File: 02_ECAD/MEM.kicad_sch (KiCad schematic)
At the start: 50 parts, among them U12 MT53E1G32D2FW-046_WT:A, U13 SDINBDG4-16G-I2, U14 IS25LP256D-JLLE

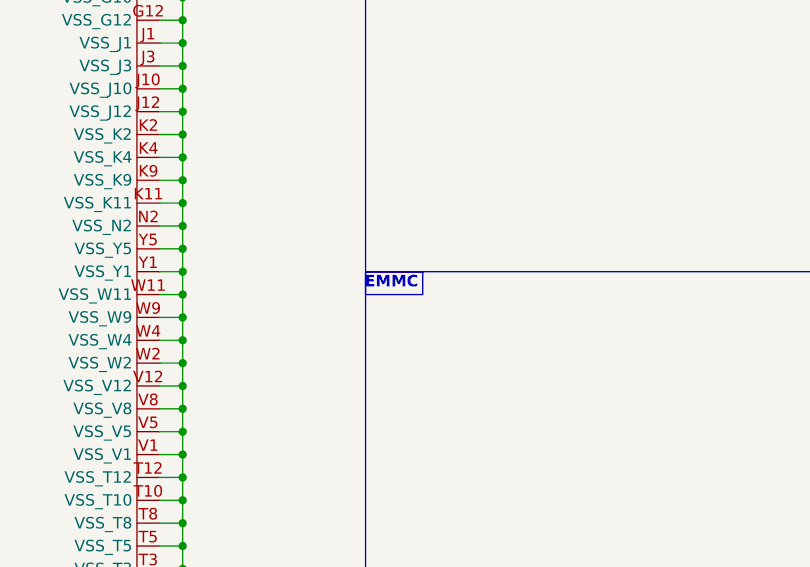
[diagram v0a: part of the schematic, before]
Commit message: Skew Check.
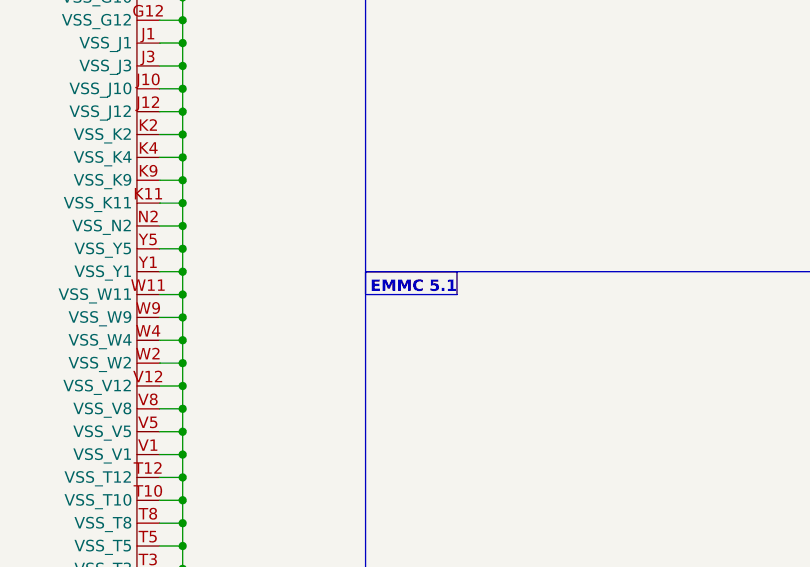
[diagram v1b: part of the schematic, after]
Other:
- note added: "EMMC 5.1"
- note removed: "EMMC"
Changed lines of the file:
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@@
 	(rectangle
 		(start 195.58 137.16)
-		(end 201.93 139.7)
+		(end 205.74 139.7)
 		(stroke
 			(width -0.0001)
@@
 		)
 	)
-	(text "EMMC"
+	(text "EMMC 5.1"
 		(exclude_from_sim no)
-		(at 201.422 139.192 0)
+		(at 205.74 139.7 0)
 		(effects
 			(font
